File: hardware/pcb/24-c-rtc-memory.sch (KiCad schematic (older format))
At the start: 10 parts, among them U701 24LC512, U702 DS1307+, Y701 CRYSTAL-32.768KHZSMD-3.2X1.5

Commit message: changed crystals
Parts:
- removed Y701: CRYSTAL-32.768KHZSMD-3.2X1.5, symbol 24-clocks-rescue:CRYSTAL-32.768KHZSMD-3.2X1.5-SparkFun-Clocks
- added Y701: 32.768kHz, Crystal:Crystal_SMD_SeikoEpson_MC306-4Pin_8.0x3.2mm, symbol Device:Crystal_GND23_Small
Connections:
- wire segments 47 -> 54
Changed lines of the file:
@@
 $EndComp
-Wire Wire Line
-	5200 5200 5200 5150
-Wire Wire Line
-	5200 5150 5400 5150
-Wire Wire Line
-	5400 5150 5400 5250
-Wire Wire Line
-	5400 5250 5500 5250
-Wire Wire Line
-	5200 5400 5200 5450
-Wire Wire Line
-	5200 5450 5400 5450
-Wire Wire Line
-	5400 5450 5400 5350
-Wire Wire Line
-	5400 5350 5500 5350
 Wire Wire Line
 	5500 5050 4750 5050
@@
 	6600 4850 6600 4950
 $Comp
-L 24-clocks-rescue:CRYSTAL-32.768KHZSMD-3.2X1.5-SparkFun-Clocks Y701
-U 1 1 5FD418B6
-P 5200 5300
-AR Path="/5FD418B6" Ref="Y701"  Part="1"
-AR Path="/5FDBDABC/5FD418B6" Ref="Y701"  Part="1"
-F 0 "Y701" V 5100 5200 45  0000 R CNN
-F 1 "CRYSTAL-32.768KHZSMD-3.2X1.5" V 5200 5200 45  0000 R CNN
-F 2 "" H 5200 5500 20  0001 C CNN
-F 3 "" H 5200 5300 50  0001 C CNN
-F 4 "XTAL-13062" V 5300 5200 60  0000 R CNN "Field4"
-F 5 "-SLAVE" H 5200 5300 50  0001 C CNN "Config"
-	1    5200 5300
-	0    1    1    0
-$EndComp
-$Comp
 L Connector:TestPoint TP701
 U 1 1 5FF95498
@@
 	6600 4400 6600 4450
 Connection ~ 6600 4450
+$Comp
+L Device:Crystal_GND23_Small Y701
+U 1 1 5FE6F3FD
+P 5200 5300
+F 0 "Y701" V 5150 5150 50  0000 R CNN
+F 1 "32.768kHz" V 5250 5150 50  0000 R CNN
+F 2 "Crystal:Crystal_SMD_SeikoEpson_MC306-4Pin_8.0x3.2mm" H 5200 5300 50  0001 C CNN
+F 3 "~" H 5200 5300 50  0001 C CNN
+	1    5200 5300
+	0    1    1    0
+$EndComp
+Wire Wire Line
+	5200 5200 5200 5150
+Wire Wire Line
+	5200 5150 5400 5150
+Wire Wire Line
+	5400 5150 5400 5250
+Wire Wire Line
+	5400 5250 5500 5250
+Wire Wire Line
+	5500 5350 5400 5350
+Wire Wire Line
+	5400 5350 5400 5450
+Wire Wire Line
+	5400 5450 5200 5450
+Wire Wire Line
+	5200 5450 5200 5400
+$Comp
+L power:GND #PWR?
+U 1 1 5FE8D112
+P 5200 5600
+F 0 "#PWR?" H 5200 5350 50  0001 C CNN
+F 1 "GND" H 5205 5427 50  0000 C CNN
+F 2 "" H 5200 5600 50  0001 C CNN
+F 3 "" H 5200 5600 50  0001 C CNN
+	1    5200 5600
+	1    0    0    -1
+$EndComp
+Wire Wire Line
+	5200 5600 5200 5550
+Wire Wire Line
+	5200 5550 5350 5550
+Wire Wire Line
+	5350 5550 5350 5300
+Wire Wire Line
+	5350 5300 5300 5300
+Wire Wire Line
+	5100 5300 5050 5300
+Wire Wire Line
+	5050 5300 5050 5550
+Wire Wire Line
+	5050 5550 5200 5550
+Connection ~ 5200 5550
 $EndSCHEMATC

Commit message: Created footprints and archived project
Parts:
- removed BT701: RC2032, symbol Device:Battery_Cell
- added BT701: CR2032, mvl-footprints:BATT_WE_79523141, symbol 24-clocks:Battery_Cell_2Plus
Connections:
- wire segments 54 -> 56
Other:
- moved on the sheet: TP703
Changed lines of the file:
@@
 L power:GND #PWR0708
 U 1 1 5FDCBDE2
-P 6600 4950
-F 0 "#PWR0708" H 6600 4700 50  0001 C CNN
-F 1 "GND" H 6605 4777 50  0000 C CNN
-F 2 "" H 6600 4950 50  0001 C CNN
-F 3 "" H 6600 4950 50  0001 C CNN
-	1    6600 4950
+P 6600 4900
+F 0 "#PWR0708" H 6600 4650 50  0001 C CNN
+F 1 "GND" H 6605 4727 50  0000 C CNN
+F 2 "" H 6600 4900 50  0001 C CNN
+F 3 "" H 6600 4900 50  0001 C CNN
+	1    6600 4900
 	1    0    0    -1
 $EndComp
@@
 	6000 4750 6000 4450
 Wire Wire Line
-	6000 4450 6600 4450
+	6000 4450 6550 4450
 Wire Wire Line
 	6000 5550 6000 5600
@@
 	3850 1250 3850 4100
 $Comp
-L Device:Battery_Cell BT701
-U 1 1 5FD3BA51
-P 6600 4750
-F 0 "BT701" H 6718 4846 50  0000 L CNN
-F 1 "RC2032" H 6718 4755 50  0000 L CNN
-F 2 "" V 6600 4810 50  0001 C CNN
-F 3 "~" V 6600 4810 50  0001 C CNN
-F 4 "-SLAVE" H 6600 4750 50  0001 C CNN "Config"
-	1    6600 4750
-	1    0    0    -1
-$EndComp
-Wire Wire Line
-	6600 4450 6600 4550
-Wire Wire Line
-	6600 4850 6600 4950
-$Comp
 L Connector:TestPoint TP701
 U 1 1 5FF95498
@@
 L Connector:TestPoint TP703
 U 1 1 5FE5017D
-P 6600 4400
-F 0 "TP703" H 6650 4500 50  0000 L CNN
-F 1 "RC2032" H 6658 4427 50  0001 L CNN
-F 2 "TestPoint:TestPoint_Pad_1.5x1.5mm" H 6800 4400 50  0001 C CNN
-F 3 "~" H 6800 4400 50  0001 C CNN
-	1    6600 4400
-	1    0    0    -1
-$EndComp
-Wire Wire Line
-	6600 4400 6600 4450
-Connection ~ 6600 4450
+P 6650 4400
+F 0 "TP703" H 6700 4500 50  0000 L CNN
+F 1 "RC2032" H 6708 4427 50  0001 L CNN
+F 2 "TestPoint:TestPoint_Pad_1.5x1.5mm" H 6850 4400 50  0001 C CNN
+F 3 "~" H 6850 4400 50  0001 C CNN
+	1    6650 4400
+	1    0    0    -1
+$EndComp
 $Comp
 L Device:Crystal_GND23_Small Y701
@@
 	5200 5450 5200 5400
 $Comp
-L power:GND #PWR?
+L power:GND #PWR0109
 U 1 1 5FE8D112
 P 5200 5600
-F 0 "#PWR?" H 5200 5350 50  0001 C CNN
+F 0 "#PWR0109" H 5200 5350 50  0001 C CNN
 F 1 "GND" H 5205 5427 50  0000 C CNN
 F 2 "" H 5200 5600 50  0001 C CNN
@@
 	5050 5550 5200 5550
 Connection ~ 5200 5550
+$Comp
+L 24-clocks:Battery_Cell_2Plus BT701
+U 1 1 5FE9121B
+P 6600 4750
+F 0 "BT701" H 6718 4871 50  0000 L CNN
+F 1 "CR2032" H 6718 4780 50  0000 L CNN
+F 2 "mvl-footprints:BATT_WE_79523141" V 6600 4810 50  0001 C CNN
+F 3 "~" V 6600 4810 50  0001 C CNN
+	1    6600 4750
+	1    0    0    -1
+$EndComp
+Wire Wire Line
+	6550 4500 6550 4450
+Connection ~ 6550 4450
+Wire Wire Line
+	6650 4450 6650 4500
+Wire Wire Line
+	6550 4450 6650 4450
+Wire Wire Line
+	6650 4400 6650 4450
+Connection ~ 6650 4450
+Wire Wire Line
+	6600 4900 6600 4850
 $EndSCHEMATC

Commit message: Added motor footprint, made init pcb
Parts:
- BT701: symbol 24-clocks:Battery_Cell_2Plus -> 24-clocks-rescue:Battery_Cell_2Plus-24-clocks
- TP701, TP702, TP703: footprint TestPoint:TestPoint_Pad_1.5x1.5mm -> TestPoint:TestPoint_Pad_D2.0mm
- U702: footprint Package_DIP:DIP-8_W7.62mm -> Package_SO:SO-8_3.9x4.9mm_P1.27mm
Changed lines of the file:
@@
 F 0 "U702" H 5600 5550 50  0000 L CNN
 F 1 "DS1307+" H 6150 4750 50  0000 L CNN
-F 2 "Package_DIP:DIP-8_W7.62mm" H 6000 4650 50  0001 C CNN
+F 2 "Package_SO:SO-8_3.9x4.9mm_P1.27mm" H 6000 4650 50  0001 C CNN
 F 3 "https://datasheets.maximintegrated.com/en/ds/DS1307.pdf" H 6000 4950 50  0001 C CNN
 F 4 "-SLAVE" H 6000 5150 50  0001 C CNN "Config"
@@
 F 0 "TP701" H 3900 1100 50  0000 L CNN
 F 1 "I2C-SDA" H 3908 1027 50  0001 L CNN
-F 2 "TestPoint:TestPoint_Pad_1.5x1.5mm" H 4050 1000 50  0001 C CNN
+F 2 "TestPoint:TestPoint_Pad_D2.0mm" H 4050 1000 50  0001 C CNN
 F 3 "~" H 4050 1000 50  0001 C CNN
 	1    3850 1000
@@
 F 0 "TP702" H 4050 1100 50  0000 L CNN
 F 1 "I2C-SCL" H 4058 1027 50  0001 L CNN
-F 2 "TestPoint:TestPoint_Pad_1.5x1.5mm" H 4200 1000 50  0001 C CNN
+F 2 "TestPoint:TestPoint_Pad_D2.0mm" H 4200 1000 50  0001 C CNN
 F 3 "~" H 4200 1000 50  0001 C CNN
 	1    4000 1000
@@
 F 0 "TP703" H 6700 4500 50  0000 L CNN
 F 1 "RC2032" H 6708 4427 50  0001 L CNN
-F 2 "TestPoint:TestPoint_Pad_1.5x1.5mm" H 6850 4400 50  0001 C CNN
+F 2 "TestPoint:TestPoint_Pad_D2.0mm" H 6850 4400 50  0001 C CNN
 F 3 "~" H 6850 4400 50  0001 C CNN
 	1    6650 4400
@@
 Connection ~ 5200 5550
 $Comp
-L 24-clocks:Battery_Cell_2Plus BT701
+L 24-clocks-rescue:Battery_Cell_2Plus-24-clocks BT701
 U 1 1 5FE9121B
 P 6600 4750

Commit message: Included all 3D files
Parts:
- BT701: Config (none) -> -SLAVE
- U701, U702: footprint Package_SO:SO-8_3.9x4.9mm_P1.27mm -> Package_SO:SOIC-8_3.9x4.9mm_P1.27mm
- Y701: footprint Crystal:Crystal_SMD_SeikoEpson_MC306-4Pin_8.0x3.2mm -> mvl-footprints:Crystal_SMD_SeikoEpson_MC306-4Pin_8.0x3.2mm; Config (none) -> -SLAVE
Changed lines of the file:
@@
 F 0 "U701" H 6600 2450 50  0000 C CNN
 F 1 "24LC512" H 6150 1850 50  0000 C CNN
-F 2 "Package_SO:SO-8_3.9x4.9mm_P1.27mm" H 6350 2150 50  0001 C CNN
+F 2 "Package_SO:SOIC-8_3.9x4.9mm_P1.27mm" H 6350 2150 50  0001 C CNN
 F 3 "http://ww1.microchip.com/downloads/en/DeviceDoc/21754M.pdf" H 6350 2150 50  0001 C CNN
 	1    6350 2150
@@
 F 0 "U702" H 5600 5550 50  0000 L CNN
 F 1 "DS1307+" H 6150 4750 50  0000 L CNN
-F 2 "Package_SO:SO-8_3.9x4.9mm_P1.27mm" H 6000 4650 50  0001 C CNN
+F 2 "Package_SO:SOIC-8_3.9x4.9mm_P1.27mm" H 6000 4650 50  0001 C CNN
 F 3 "https://datasheets.maximintegrated.com/en/ds/DS1307.pdf" H 6000 4950 50  0001 C CNN
 F 4 "-SLAVE" H 6000 5150 50  0001 C CNN "Config"
@@
 F 0 "Y701" V 5150 5150 50  0000 R CNN
 F 1 "32.768kHz" V 5250 5150 50  0000 R CNN
-F 2 "Crystal:Crystal_SMD_SeikoEpson_MC306-4Pin_8.0x3.2mm" H 5200 5300 50  0001 C CNN
+F 2 "mvl-footprints:Crystal_SMD_SeikoEpson_MC306-4Pin_8.0x3.2mm" H 5200 5300 50  0001 C CNN
 F 3 "~" H 5200 5300 50  0001 C CNN
+F 4 "-SLAVE" H 5200 5300 50  0001 C CNN "Config"
 	1    5200 5300
 	0    1    1    0
@@
 F 2 "mvl-footprints:BATT_WE_79523141" V 6600 4810 50  0001 C CNN
 F 3 "~" V 6600 4810 50  0001 C CNN
+F 4 "-SLAVE" H 6600 4750 50  0001 C CNN "Config"
 	1    6600 4750
 	1    0    0    -1

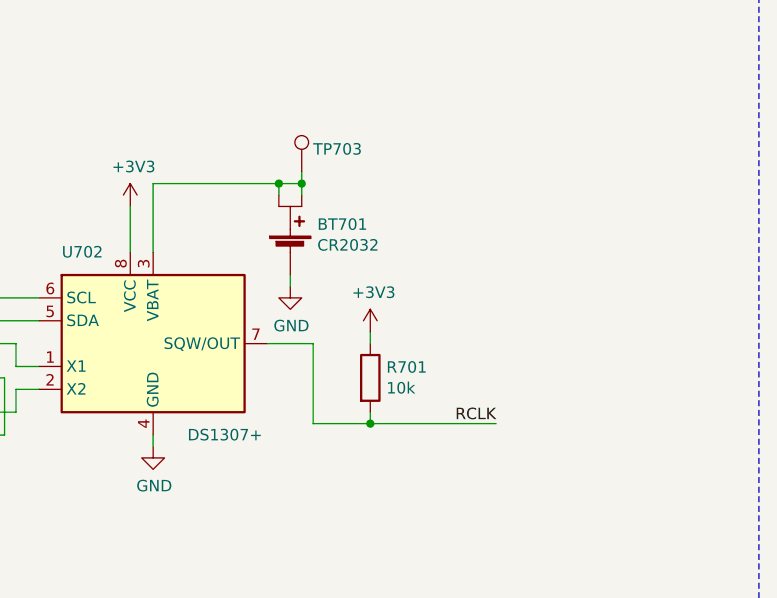
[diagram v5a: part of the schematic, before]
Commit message: Added routing
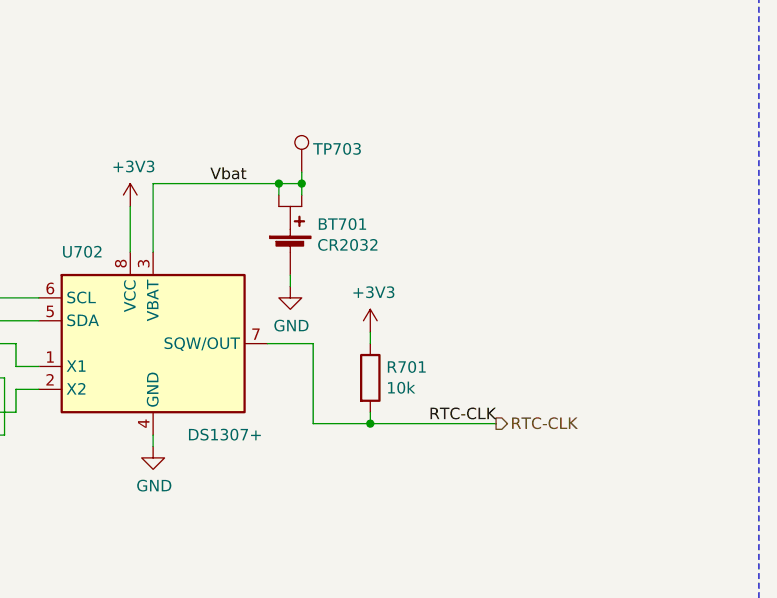
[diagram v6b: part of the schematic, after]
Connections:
- net Vbat: now reaches BT701.1 (+), BT701.3 (+), TP703.1, U702.3 (VBAT)
- net RCLK renamed RTC-CLK
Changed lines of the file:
@@
 Connection ~ 6950 5500
 Text Label 7500 5500 2    50   ~ 0
-RCLK
+RTC-CLK
 Wire Wire Line
 	5900 4550 5900 4750
@@
 Wire Wire Line
 	6600 4900 6600 4850
+Text Label 6250 4450 0    50   ~ 0
+Vbat
+Text HLabel 7500 5500 2    50   Output ~ 0
+RTC-CLK
 $EndSCHEMATC

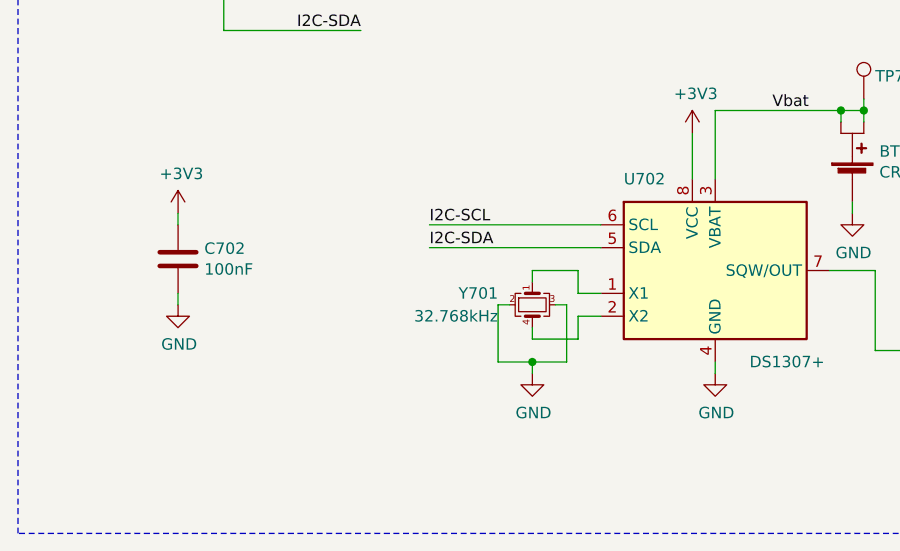
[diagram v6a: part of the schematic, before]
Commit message: Finished routing
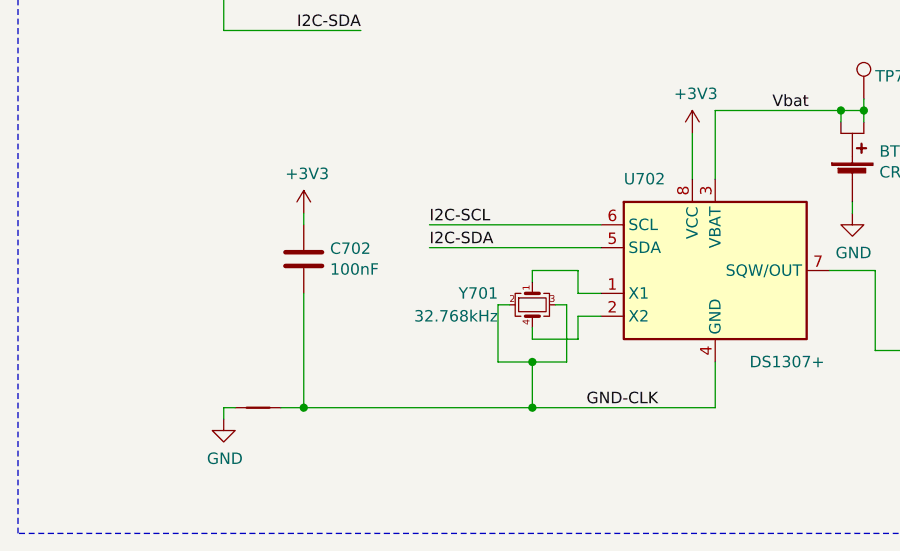
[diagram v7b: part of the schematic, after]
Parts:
- added NT701: Net-Tie_2, NetTie:NetTie-2_SMD_Pad0.5mm, symbol Device:Net-Tie_2
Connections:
- net GND: now also NT701.2; no longer C702.2, U702.4 (GND), Y701.2, Y701.3
- new net GND-CLK: C702.2, NT701.1, U702.4 (GND), Y701.2, Y701.3
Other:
- moved on the sheet: C702
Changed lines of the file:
@@
 L power:GND #PWR0711
 U 1 1 5FDCBDE8
-P 6000 5600
-F 0 "#PWR0711" H 6000 5350 50  0001 C CNN
-F 1 "GND" H 6005 5427 50  0000 C CNN
-F 2 "" H 6000 5600 50  0001 C CNN
-F 3 "" H 6000 5600 50  0001 C CNN
-	1    6000 5600
+P 3850 5800
+F 0 "#PWR0711" H 3850 5550 50  0001 C CNN
+F 1 "GND" H 3855 5627 50  0000 C CNN
+F 2 "" H 3850 5800 50  0001 C CNN
+F 3 "" H 3850 5800 50  0001 C CNN
+	1    3850 5800
 	1    0    0    -1
 $EndComp
@@
 	6000 4450 6550 4450
 Wire Wire Line
-	6000 5550 6000 5600
-Wire Wire Line
 	6950 5500 7500 5500
 Connection ~ 6950 5500
@@
 L Device:C C702
 U 1 1 5FDCBDFD
-P 3650 5100
-F 0 "C702" H 3765 5146 50  0000 L CNN
-F 1 "100nF" H 3765 5055 50  0000 L CNN
-F 2 "Capacitor_SMD:C_0603_1608Metric" H 3688 4950 50  0001 C CNN
-F 3 "~" H 3650 5100 50  0001 C CNN
-F 4 "-SLAVE" H 3650 5100 50  0001 C CNN "Config"
-	1    3650 5100
-	1    0    0    -1
-$EndComp
-$Comp
-L power:GND #PWR0710
-U 1 1 5FDCBE03
-P 3650 5300
-F 0 "#PWR0710" H 3650 5050 50  0001 C CNN
-F 1 "GND" H 3655 5127 50  0000 C CNN
-F 2 "" H 3650 5300 50  0001 C CNN
-F 3 "" H 3650 5300 50  0001 C CNN
-	1    3650 5300
+P 4200 5100
+F 0 "C702" H 4315 5146 50  0000 L CNN
+F 1 "100nF" H 4315 5055 50  0000 L CNN
+F 2 "Capacitor_SMD:C_0603_1608Metric" H 4238 4950 50  0001 C CNN
+F 3 "~" H 4200 5100 50  0001 C CNN
+F 4 "-SLAVE" H 4200 5100 50  0001 C CNN "Config"
+	1    4200 5100
 	1    0    0    -1
 $EndComp
@@
 L power:+3V3 #PWR0707
 U 1 1 5FDCBE09
-P 3650 4900
-F 0 "#PWR0707" H 3650 4750 50  0001 C CNN
-F 1 "+3V3" H 3665 5073 50  0000 C CNN
-F 2 "" H 3650 4900 50  0001 C CNN
-F 3 "" H 3650 4900 50  0001 C CNN
-	1    3650 4900
-	1    0    0    -1
-$EndComp
-Wire Wire Line
-	3650 4900 3650 4950
-Wire Wire Line
-	3650 5250 3650 5300
+P 4200 4900
+F 0 "#PWR0707" H 4200 4750 50  0001 C CNN
+F 1 "+3V3" H 4215 5073 50  0000 C CNN
+F 2 "" H 4200 4900 50  0001 C CNN
+F 3 "" H 4200 4900 50  0001 C CNN
+	1    4200 4900
+	1    0    0    -1
+$EndComp
+Wire Wire Line
+	4200 4900 4200 4950
 Text Label 4450 3950 2    50   ~ 0
 I2C-SCL
@@
 Wire Wire Line
 	5200 5450 5200 5400
-$Comp
-L power:GND #PWR0109
-U 1 1 5FE8D112
-P 5200 5600
-F 0 "#PWR0109" H 5200 5350 50  0001 C CNN
-F 1 "GND" H 5205 5427 50  0000 C CNN
-F 2 "" H 5200 5600 50  0001 C CNN
-F 3 "" H 5200 5600 50  0001 C CNN
-	1    5200 5600
-	1    0    0    -1
-$EndComp
-Wire Wire Line
-	5200 5600 5200 5550
 Wire Wire Line
 	5200 5550 5350 5550
@@
 Text HLabel 7500 5500 2    50   Output ~ 0
 RTC-CLK
+$Comp
+L Device:Net-Tie_2 NT701
+U 1 1 601FC6FC
+P 4000 5750
+F 0 "NT701" V 3954 5794 50  0001 L CNN
+F 1 "Net-Tie_2" V 4045 5794 50  0001 L CNN
+F 2 "NetTie:NetTie-2_SMD_Pad0.5mm" H 4000 5750 50  0001 C CNN
+F 3 "~" H 4000 5750 50  0001 C CNN
+	1    4000 5750
+	-1   0    0    1
+$EndComp
+Text Label 5750 5750 2    50   ~ 0
+GND-CLK
+Wire Wire Line
+	3850 5800 3850 5750
+Wire Wire Line
+	3850 5750 3900 5750
+Wire Wire Line
+	6000 5550 6000 5750
+Wire Wire Line
+	5200 5550 5200 5750
+Connection ~ 5200 5750
+Wire Wire Line
+	5200 5750 6000 5750
+Wire Wire Line
+	4200 5750 5200 5750
+Wire Wire Line
+	4200 5250 4200 5750
+Wire Wire Line
+	4100 5750 4200 5750
+Connection ~ 4200 5750
 $EndSCHEMATC
